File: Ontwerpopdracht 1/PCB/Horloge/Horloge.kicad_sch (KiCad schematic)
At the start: 49 parts, among them J1 Conn_01x03, Q1 BSS138, U1 TPS613222ADBVT, U2 ATTINY414-SSF, Y1 FX135A-327

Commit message: pcb finaal + code
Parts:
- J1: footprint Connector_PinHeader_1.00mm:PinHeader_1x03_P1.00mm_Vertical -> Connector_PinHeader_2.54mm:PinHeader_1x03_P2.54mm_Vertical
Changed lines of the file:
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@@
       (effects (font (size 1.27 1.27)) (justify left) hide)
     )
-    (property "Footprint" "Connector_PinHeader_1.00mm:PinHeader_1x03_P1.00mm_Vertical" (id 2) (at 31.75 57.15 0)
+    (property "Footprint" "Connector_PinHeader_2.54mm:PinHeader_1x03_P2.54mm_Vertical" (id 2) (at 31.75 57.15 0)
       (effects (font (size 1.27 1.27)) hide)
     )
@@
     )
     (path "/35d1ac95-96f8-4902-9ae0-f86acb453796"
-      (reference "J1") (unit 1) (value "Conn_01x03") (footprint "Connector_PinHeader_1.00mm:PinHeader_1x03_P1.00mm_Vertical")
+      (reference "J1") (unit 1) (value "Conn_01x03") (footprint "Connector_PinHeader_2.54mm:PinHeader_1x03_P2.54mm_Vertical")
     )
     (path "/e8b02372-df70-4a53-bb2e-192ce2085ac9"

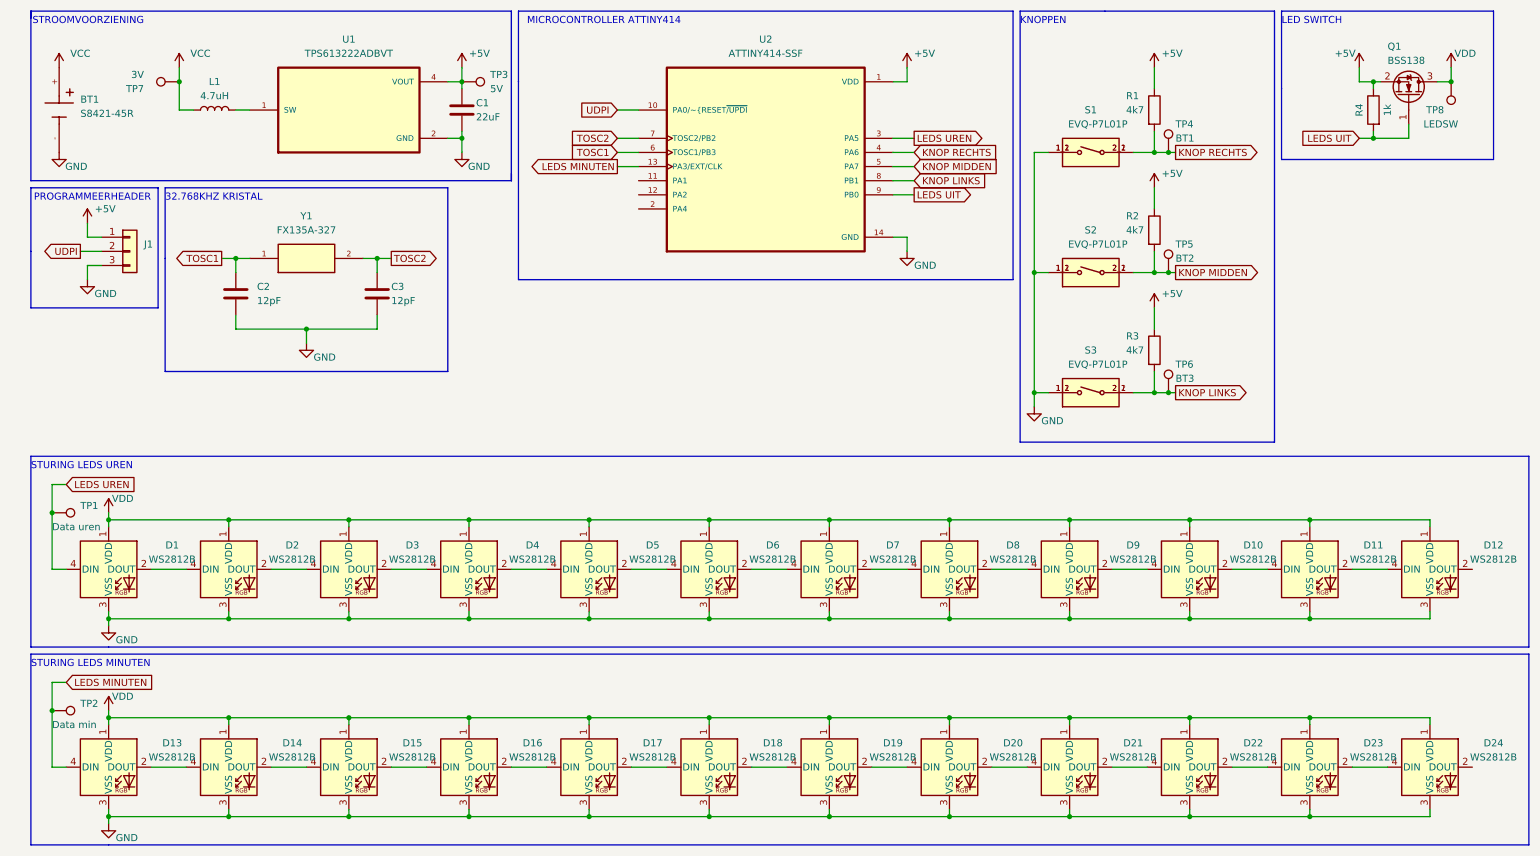
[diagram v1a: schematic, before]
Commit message: pcb macropad klaar
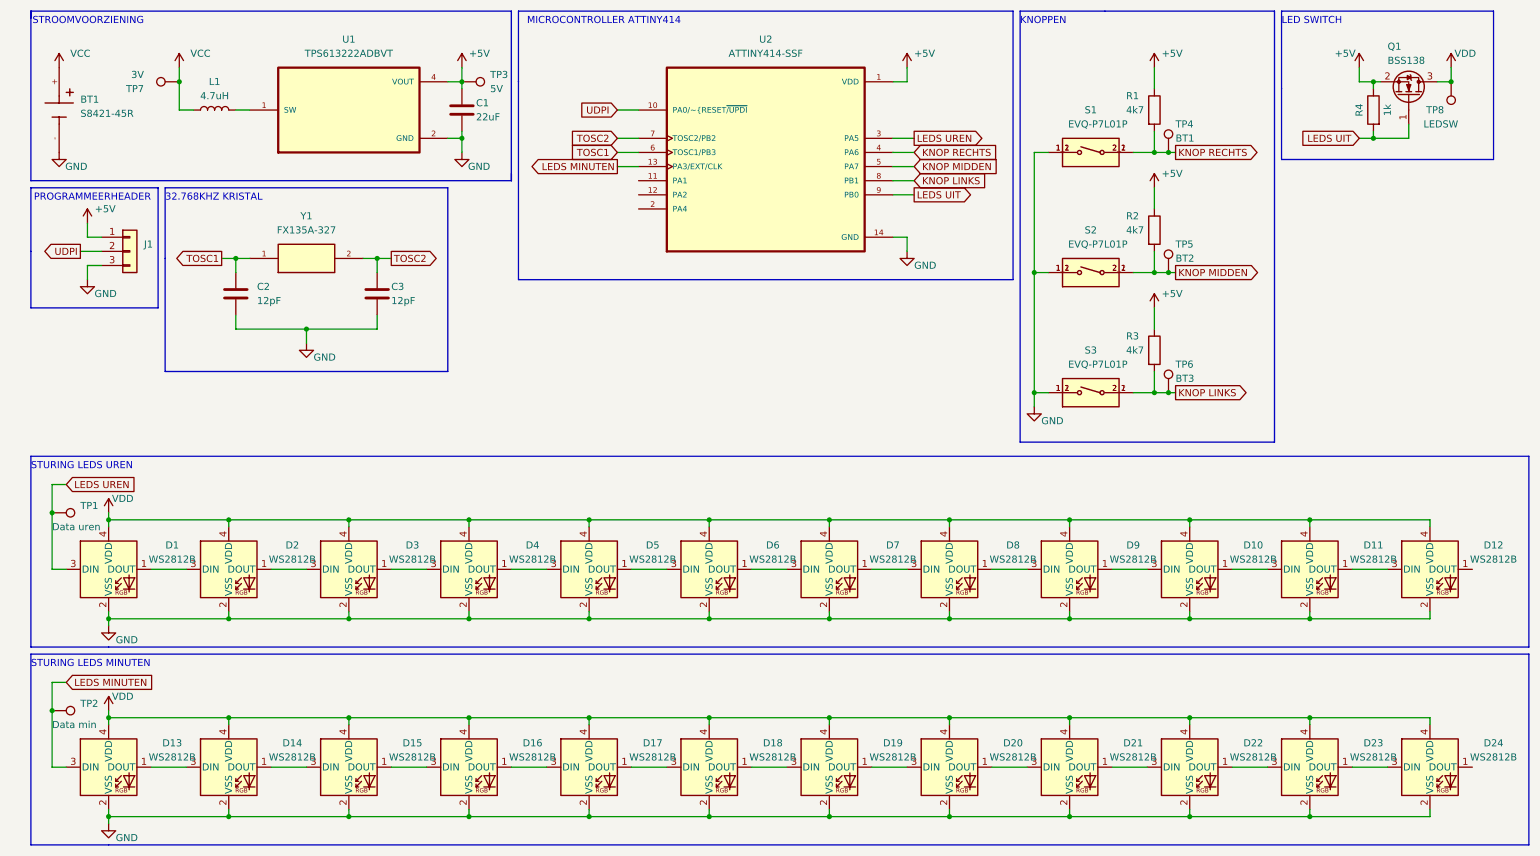
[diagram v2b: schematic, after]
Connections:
- net GND: now also D1.2 (VSS), D10.2 (VSS), D11.2 (VSS), D12.2 (VSS), D13.2 (VSS), D14.2 (VSS), D15.2 (VSS), D16.2 (VSS), D17.2 (VSS), D18.2 (VSS), D19.2 (VSS), D2.2 (VSS), D20.2 (VSS), D21.2 (VSS), D22.2 (VSS), D23.2 (VSS), D24.2 (VSS), D3.2 (VSS), D4.2 (VSS), D5.2 (VSS), D6.2 (VSS), D7.2 (VSS), D8.2 (VSS), D9.2 (VSS); no longer D1.3 (VSS), D10.3 (VSS), D11.3 (VSS), D12.3 (VSS), D13.3 (VSS), D14.3 (VSS), D15.3 (VSS), D16.3 (VSS), D17.3 (VSS), D18.3 (VSS), D19.3 (VSS), D2.3 (VSS), D20.3 (VSS), D21.3 (VSS), D22.3 (VSS), D23.3 (VSS), D24.3 (VSS), D3.3 (VSS), D4.3 (VSS), D5.3 (VSS), D6.3 (VSS), D7.3 (VSS), D8.3 (VSS), D9.3 (VSS)
- net LEDS MINUTEN: now also D13.3 (DIN); no longer D13.4 (DIN)
- net LEDS UREN: now also D1.3 (DIN); no longer D1.4 (DIN)
- net VDD: now also D1.4 (VDD), D10.4 (VDD), D11.4 (VDD), D12.4 (VDD), D13.4 (VDD), D14.4 (VDD), D15.4 (VDD), D16.4 (VDD), D17.4 (VDD), D18.4 (VDD), D19.4 (VDD), D2.4 (VDD), D20.4 (VDD), D21.4 (VDD), D22.4 (VDD), D23.4 (VDD), D24.4 (VDD), D3.4 (VDD), D4.4 (VDD), D5.4 (VDD), D6.4 (VDD), D7.4 (VDD), D8.4 (VDD), D9.4 (VDD); no longer D1.1 (VDD), D10.1 (VDD), D11.1 (VDD), D12.1 (VDD), D13.1 (VDD), D14.1 (VDD), D15.1 (VDD), D16.1 (VDD), D17.1 (VDD), D18.1 (VDD), D19.1 (VDD), D2.1 (VDD), D20.1 (VDD), D21.1 (VDD), D22.1 (VDD), D23.1 (VDD), D24.1 (VDD), D3.1 (VDD), D4.1 (VDD), D5.1 (VDD), D6.1 (VDD), D7.1 (VDD), D8.1 (VDD), D9.1 (VDD)
- new net: D20.1 (DOUT), D21.3 (DIN)
- new net: D19.1 (DOUT), D20.3 (DIN)
- new net: D4.1 (DOUT), D5.3 (DIN)
- new net: D3.1 (DOUT), D4.3 (DIN)
- new net: D11.1 (DOUT), D12.3 (DIN)
- new net: D10.1 (DOUT), D11.3 (DIN)
- new net: D23.1 (DOUT), D24.3 (DIN)
- new net: D18.1 (DOUT), D19.3 (DIN)
- new net: D17.1 (DOUT), D18.3 (DIN)
- new net: D2.1 (DOUT), D3.3 (DIN)
- new net: D1.1 (DOUT), D2.3 (DIN)
- new net: D22.1 (DOUT), D23.3 (DIN)
- new net: D21.1 (DOUT), D22.3 (DIN)
- new net: D7.1 (DOUT), D8.3 (DIN)
- new net: D6.1 (DOUT), D7.3 (DIN)
- new net: D13.1 (DOUT), D14.3 (DIN)
- new net: D16.1 (DOUT), D17.3 (DIN)
- new net: D14.1 (DOUT), D15.3 (DIN)
- new net: D10.3 (DIN), D9.1 (DOUT)
- new net: D8.1 (DOUT), D9.3 (DIN)
- new net: D5.1 (DOUT), D6.3 (DIN)
- new net: D15.1 (DOUT), D16.3 (DIN)
